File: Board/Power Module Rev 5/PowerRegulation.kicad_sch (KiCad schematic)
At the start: 8 parts, among them U14 TPS2116DRLR, U15 NCP167BMX330TBG

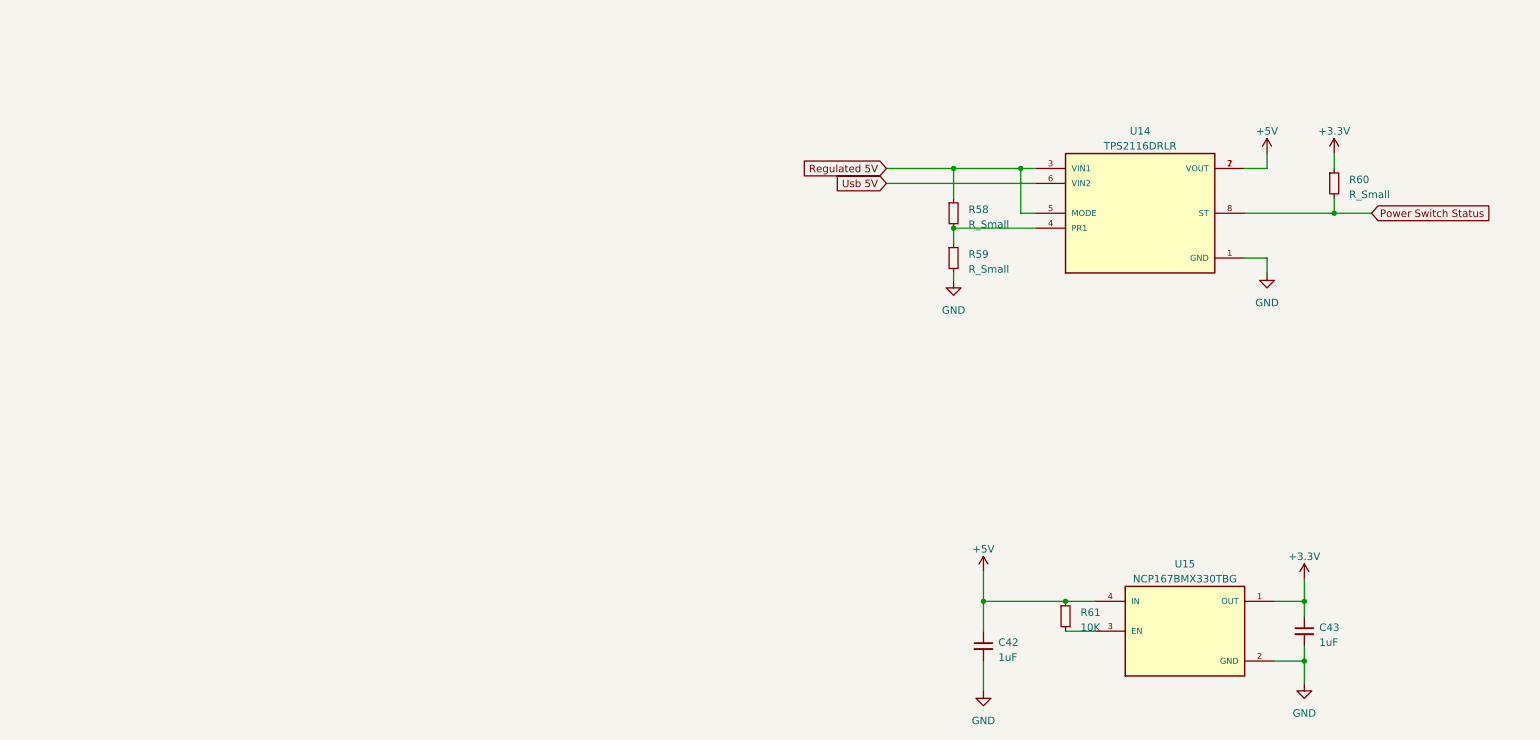
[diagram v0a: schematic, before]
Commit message: Board Progress
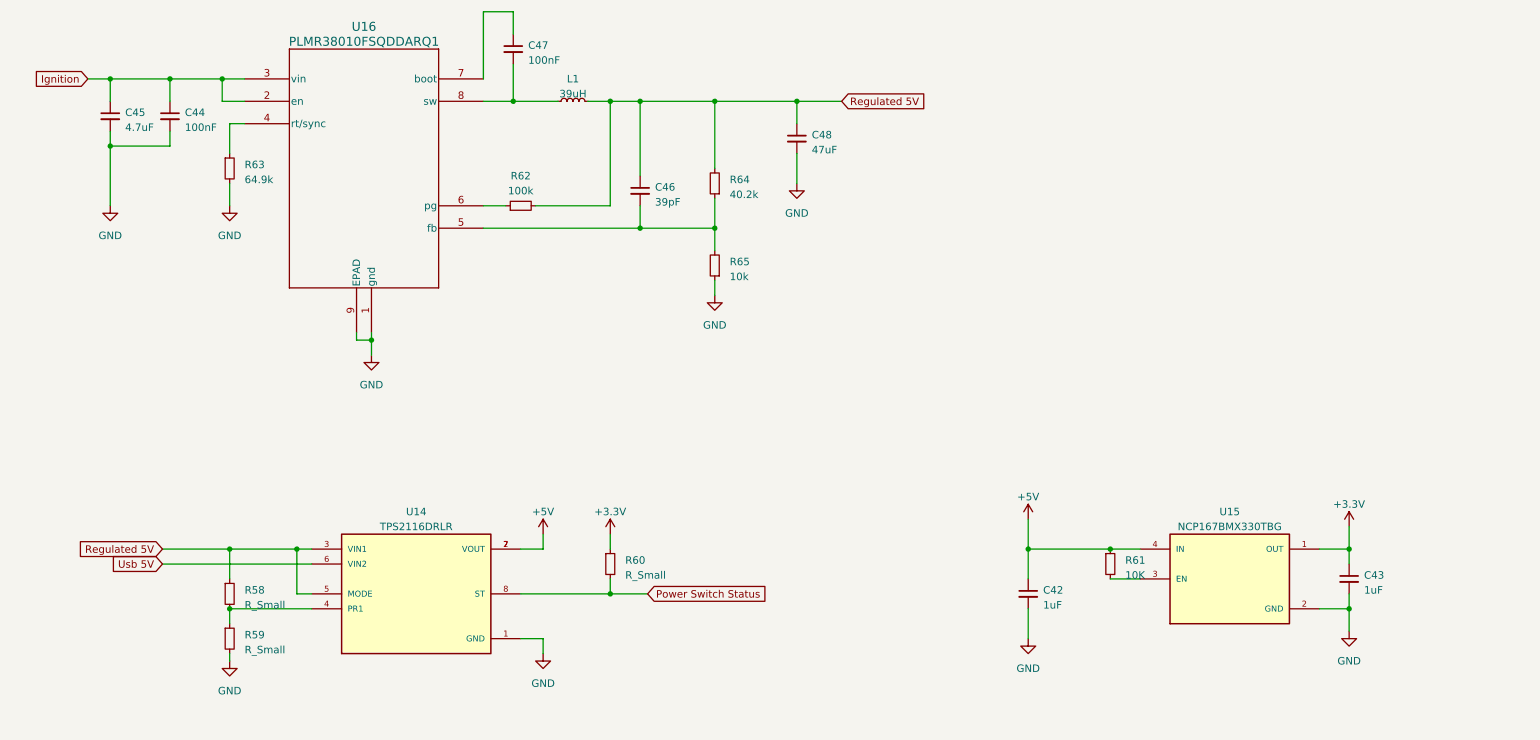
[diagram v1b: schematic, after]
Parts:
- added C44, C47: 100nF, Capacitor_SMD:C_0603_1608Metric_Pad1.08x0.95mm_HandSolder, symbol Device:C_Small
- added C45: 4.7uF, Capacitor_SMD:C_1210_3225Metric_Pad1.33x2.70mm_HandSolder, symbol Device:C_Small
- added C46: 39pF, Capacitor_SMD:C_0603_1608Metric_Pad1.08x0.95mm_HandSolder, symbol Device:C_Small
- added C48: 47uF, Capacitor_SMD:C_1210_3225Metric_Pad1.33x2.70mm_HandSolder, symbol Device:C_Small
- added L1: 39uH, Inductor_SMD:L_Wuerth_WE-PD-Typ-LS, symbol Device:L_Small
- added R62: 100k, Resistor_SMD:R_0603_1608Metric_Pad0.98x0.95mm_HandSolder, symbol Device:R_Small
- added R63: 64.9k, Resistor_SMD:R_0603_1608Metric_Pad0.98x0.95mm_HandSolder, symbol Device:R_Small
- added R64: 40.2k, Resistor_SMD:R_0603_1608Metric_Pad0.98x0.95mm_HandSolder, symbol Device:R_Small
- added R65: 10k, Resistor_SMD:R_0603_1608Metric_Pad0.98x0.95mm_HandSolder, symbol Device:R_Small
- added U16: PLMR38010FSQDDARQ1, MyKiCadLibraries:HSOP8_DDA_TEX, symbol MyLibrary:PLMR38010FSQDDARQ1
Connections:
- net EPAD: now also C44.2, C45.2, C48.2, R63.2, R65.1, U16.1 (gnd), U16.9 (EPAD)
- net Regulated 5V: now also C46.1, C48.1, L1.2, R62.2, R64.2
- new net: R62.1, U16.6 (pg)
- new net: R63.1, U16.4 (rt/sync)
- new net: C46.2, R64.1, R65.2, U16.5 (fb)
- new net: C47.1, U16.7 (boot)
- new net: C47.2, L1.1, U16.8 (sw)
- new net Ignition: C44.1, C45.1, U16.2 (en), U16.3 (vin)
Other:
- moved on the sheet: C42, C43, R58, R59, R60, R61, U14, U15

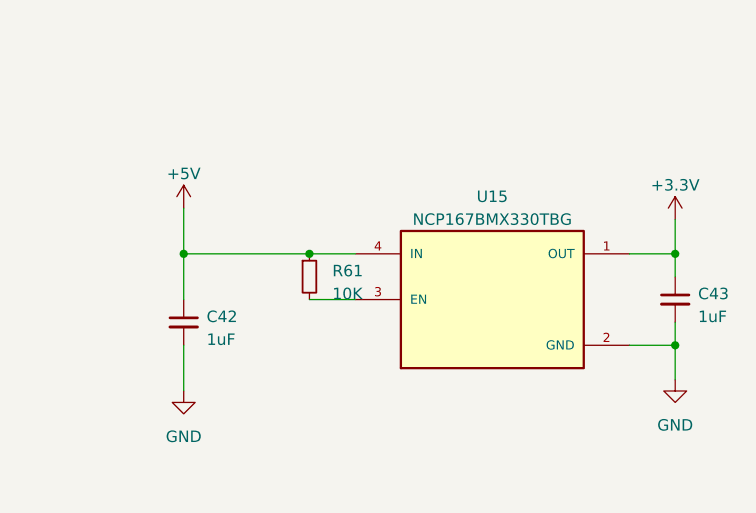
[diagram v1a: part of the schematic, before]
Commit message: Board Update
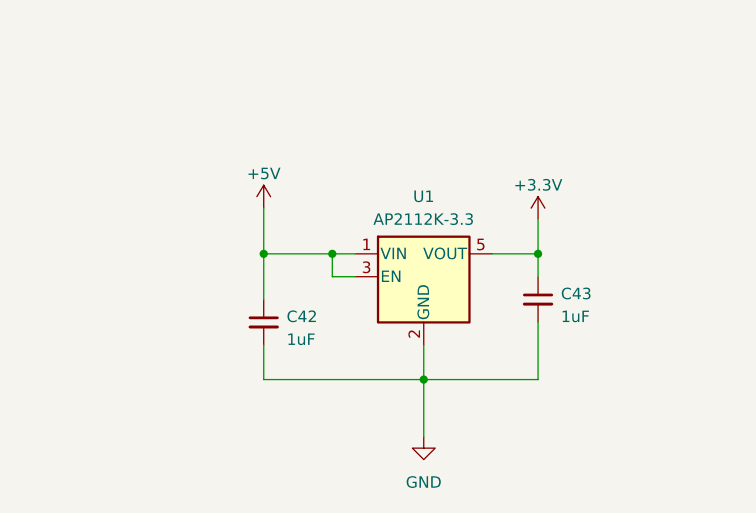
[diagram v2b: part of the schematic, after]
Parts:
- removed R61: 10K, Resistor_SMD:R_0603_1608Metric_Pad0.98x0.95mm_HandSolder, symbol Device:R_Small
- removed U15: NCP167BMX330TBG, Package_DFN_QFN:OnSemi_XDFN4-1EP_1.0x1.0mm_EP0.52x0.52mm, symbol MyLibrary:NCP167BMX330TBG
- added U1: AP2112K-3.3, Package_TO_SOT_SMD:SOT-23-5, symbol Regulator_Linear:AP2112K-3.3
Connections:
- net +3.3V: now also U1.5 (VOUT)
- net +5V: now also U1.1 (VIN), U1.3 (EN)
- net EPAD renamed GND
- net GND: now also U1.2 (GND)
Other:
- moved on the sheet: C42, C43
